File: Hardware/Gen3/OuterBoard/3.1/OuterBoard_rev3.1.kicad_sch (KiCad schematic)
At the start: 103 parts, among them J1 6130XX11121_61300611121, J3 F32R-1A7H1-11024, J42 UJ31-CH-G2-SMT-TR, J7 530470210, J8 530470210, SW1 PTS815 SJM 250 SMTR LFS, SW2 PTS815 SJM 250 SMTR LFS, U11 GD25Q64CSIGR, U2 BNO055, U2 MCP73812T-420I-OT, U3 MCP73812T-420I-OT, U3 MIC5504-3.3YM5, U5 MIC5504-1.8YM5, U6 MCP1700x-280xxTT, U7 ESP32-S3, Y1 ABM8G-40.000MHZ-18-D2Y-T

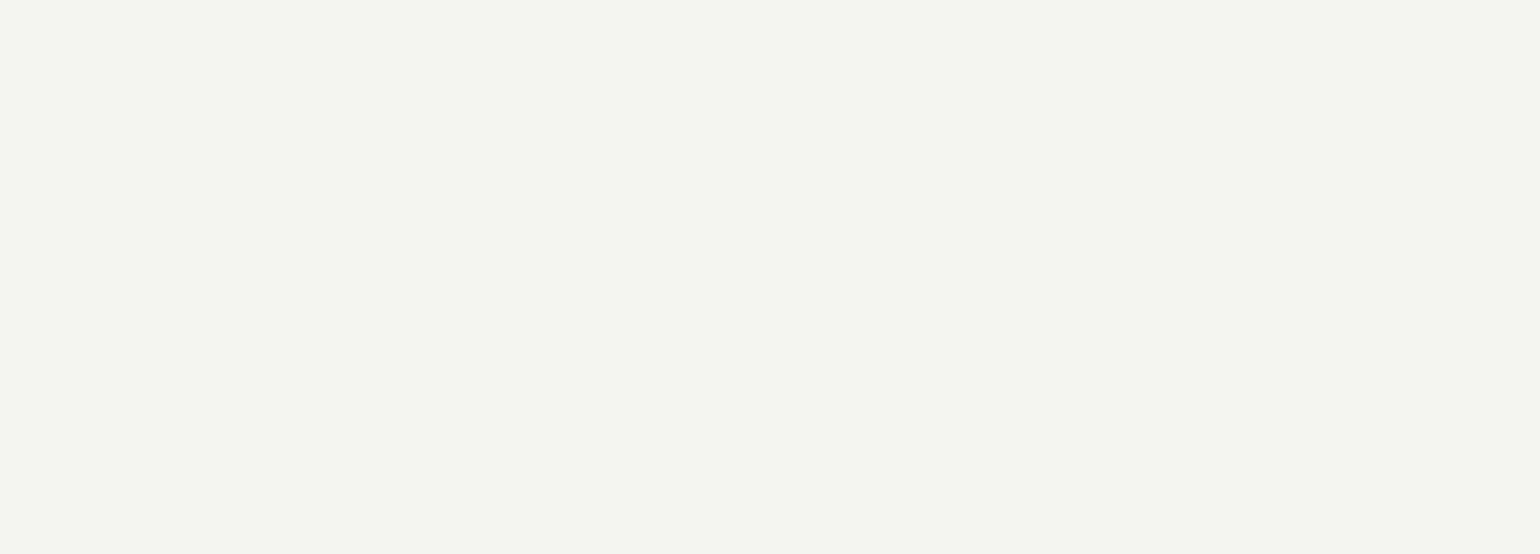
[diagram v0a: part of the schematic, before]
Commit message: wait for testing result
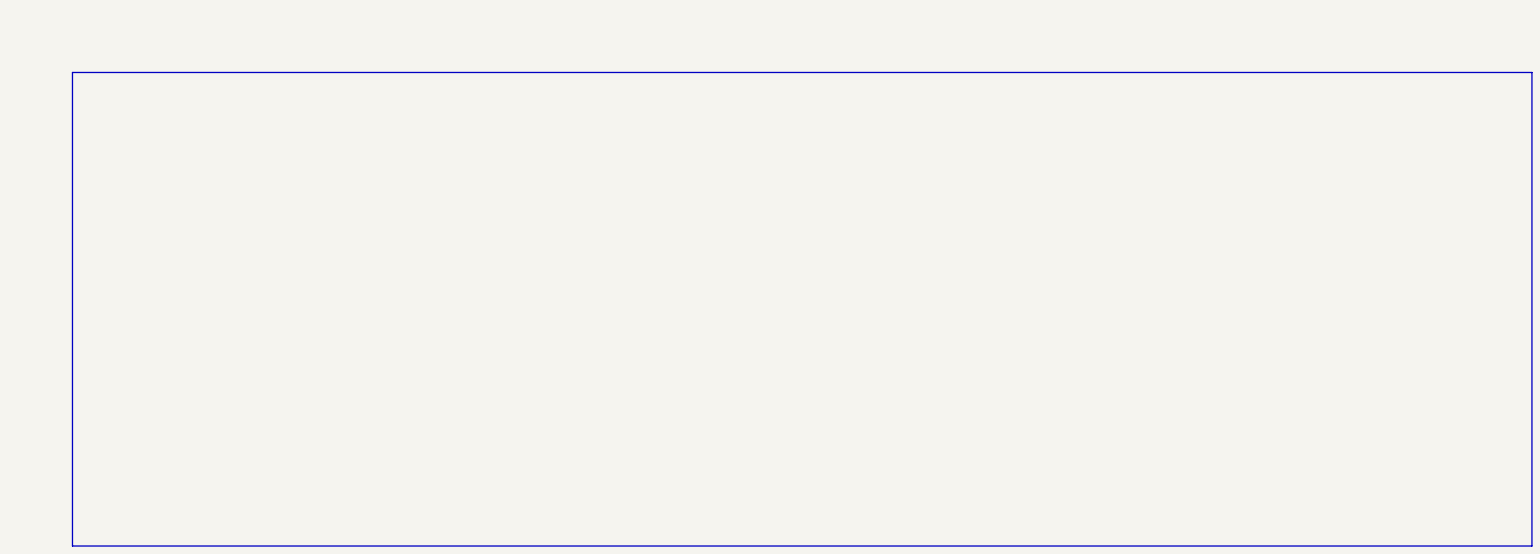
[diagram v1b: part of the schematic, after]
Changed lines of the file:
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@@
+	)
+	(rectangle
+		(start 648.335 312.42)
+		(end 1010.793 430.022)
+		(stroke
+			(width 0)
+			(type default)
+		)
+		(fill
+			(type none)
+		)
 	)
 	(rectangle
